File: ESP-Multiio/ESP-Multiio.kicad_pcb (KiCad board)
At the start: 2 copper layers, 75 x 59 mm, 50 parts, among them J1 Conn_01x10, Q1 BC337, SW1 SW_SPDT_MSM, SW2 SW_SPDT_MSM, SW3 SW_SPDT_MSM, SW4 SW_SPDT_MSM, U1 WeMos_D1_mini, U2 MCP23017_SP, U4 TSOP1838

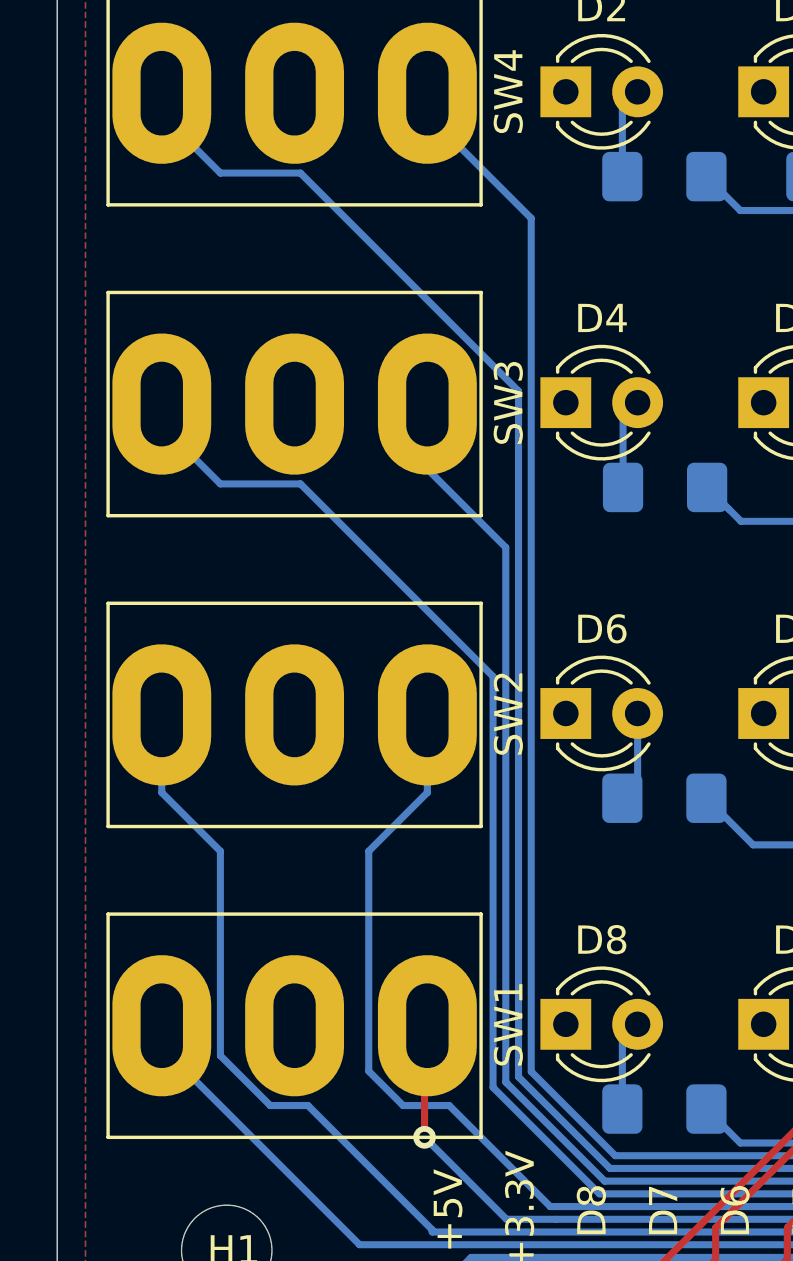
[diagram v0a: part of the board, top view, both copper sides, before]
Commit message: more 3.3V fill
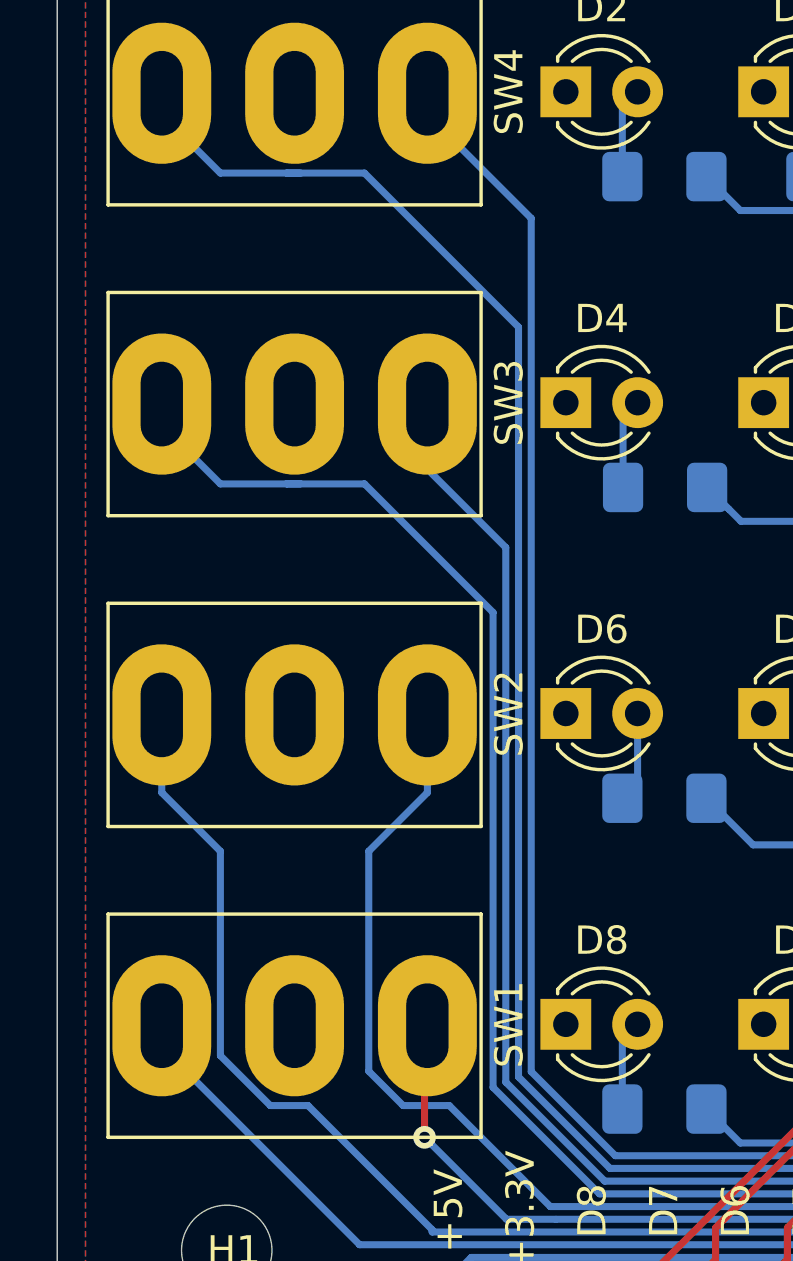
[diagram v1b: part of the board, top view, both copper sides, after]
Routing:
- net /GPB6: track 100.9 -> 102.7 mm
- net /GPB4: track 94.2 -> 96.0 mm
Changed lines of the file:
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@@
     (thickness 1.6)
     (drawings 51)
-    (tracks 363)
+    (tracks 367)
     (zones 0)
     (modules 50)
@@
     (add_net "Net-(Q1-Pad1)")
     (add_net "Net-(Q1-Pad2)")
-    (add_net "Net-(U2-Pad11)")
-    (add_net "Net-(U2-Pad14)")
     (add_net SCL)
     (add_net SDA)
@@
   (segment (start 80.7 51.8) (end 80.7 51.05) (width 0.25) (layer B.Cu) (net 42))
   (segment (start 82.77501 53.87501) (end 80.7 51.8) (width 0.25) (layer B.Cu) (net 42))
-  (segment (start 92.424972 75.234892) (end 92.424972 60.690465) (width 0.25) (layer B.Cu) (net 42))
+  (segment (start 87.87501 53.87501) (end 85.12499 53.87501) (width 0.25) (layer B.Cu) (net 42))
+  (segment (start 92.424972 75.234892) (end 92.424972 58.424972) (width 0.25) (layer B.Cu) (net 42))
+  (segment (start 92.424972 58.424972) (end 87.87501 53.87501) (width 0.25) (layer B.Cu) (net 42))
   (segment (start 96.19013 79.00005) (end 92.424972 75.234892) (width 0.25) (layer B.Cu) (net 42))
-  (segment (start 112.61259 75.80874) (end 109.42128 79.00005) (width 0.25) (layer B.Cu) (net 42))
+  (segment (start 109.42128 79.00005) (end 96.19013 79.00005) (width 0.25) (layer B.Cu) (net 42))
+  (segment (start 112.61259 68.836406) (end 112.61259 75.80874) (width 0.25) (layer B.Cu) (net 42))
+  (segment (start 85.12499 53.87501) (end 82.77501 53.87501) (width 0.25) (layer B.Cu) (net 42))
+  (segment (start 85.609517 53.87501) (end 85.12499 53.87501) (width 0.25) (layer B.Cu) (net 42))
+  (segment (start 118.065994 64.42501) (end 117.023986 64.42501) (width 0.25) (layer B.Cu) (net 42))
   (segment (start 135.84 45.62) (end 135.040001 46.419999) (width 0.25) (layer B.Cu) (net 42))
+  (segment (start 112.61259 75.80874) (end 109.42128 79.00005) (width 0.25) (layer B.Cu) (net 42))
   (segment (start 135.040001 46.419999) (end 135.040001 47.451003) (width 0.25) (layer B.Cu) (net 42))
-  (segment (start 85.609517 53.87501) (end 82.77501 53.87501) (width 0.25) (layer B.Cu) (net 42))
-  (segment (start 135.040001 47.451003) (end 118.065994 64.42501) (width 0.25) (layer B.Cu) (net 42))
   (segment (start 117.023986 64.42501) (end 112.61259 68.836406) (width 0.25) (layer B.Cu) (net 42))
-  (segment (start 92.424972 60.690465) (end 85.609517 53.87501) (width 0.25) (layer B.Cu) (net 42))
-  (segment (start 118.065994 64.42501) (end 117.023986 64.42501) (width 0.25) (layer B.Cu) (net 42))
-  (segment (start 109.42128 79.00005) (end 96.19013 79.00005) (width 0.25) (layer B.Cu) (net 42))
-  (segment (start 112.61259 68.836406) (end 112.61259 75.80874) (width 0.25) (layer B.Cu) (net 42))
+  (segment (start 135.040001 47.451003) (end 118.065994 64.42501) (width 0.25) (layer B.Cu) (net 42))
   (segment (start 92.874981 75.048491) (end 92.874981 56.124981) (width 0.25) (layer B.Cu) (net 43))
   (segment (start 92.874981 56.124981) (end 90 53.25) (width 0.25) (layer B.Cu) (net 43))
@@
   (segment (start 112.16258 66.746416) (end 117.023986 61.88501) (width 0.25) (layer B.Cu) (net 43))
   (segment (start 82.77501 42.87501) (end 80.7 40.8) (width 0.25) (layer B.Cu) (net 44))
-  (segment (start 93.32499 50.590483) (end 85.609517 42.87501) (width 0.25) (layer B.Cu) (net 44))
-  (segment (start 96.56293 78.10003) (end 93.32499 74.86209) (width 0.25) (layer B.Cu) (net 44))
-  (segment (start 93.32499 74.86209) (end 93.32499 50.590483) (width 0.25) (layer B.Cu) (net 44))
+  (segment (start 80.7 40.8) (end 80.7 40.05) (width 0.25) (layer B.Cu) (net 44))
+  (segment (start 87.87501 42.87501) (end 85.12499 42.87501) (width 0.25) (layer B.Cu) (net 44))
+  (segment (start 93.32499 74.86209) (end 93.32499 48.32499) (width 0.25) (layer B.Cu) (net 44))
   (segment (start 109.04848 78.10003) (end 96.56293 78.10003) (width 0.25) (layer B.Cu) (net 44))
+  (segment (start 111.71257 64.656426) (end 111.71257 75.43594) (width 0.25) (layer B.Cu) (net 44))
+  (segment (start 117.023986 59.34501) (end 111.71257 64.656426) (width 0.25) (layer B.Cu) (net 44))
+  (segment (start 85.12499 42.87501) (end 82.77501 42.87501) (width 0.25) (layer B.Cu) (net 44))
+  (segment (start 118.065994 59.34501) (end 117.023986 59.34501) (width 0.25) (layer B.Cu) (net 44))
+  (segment (start 96.56293 78.10003) (end 93.32499 74.86209) (width 0.25) (layer B.Cu) (net 44))
+  (segment (start 129.960001 46.419999) (end 129.960001 47.451003) (width 0.25) (layer B.Cu) (net 44))
+  (segment (start 85.609517 42.87501) (end 85.12499 42.87501) (width 0.25) (layer B.Cu) (net 44))
   (segment (start 111.71257 75.43594) (end 109.04848 78.10003) (width 0.25) (layer B.Cu) (net 44))
   (segment (start 130.76 45.62) (end 129.960001 46.419999) (width 0.25) (layer B.Cu) (net 44))
+  (segment (start 93.32499 48.32499) (end 87.87501 42.87501) (width 0.25) (layer B.Cu) (net 44))
   (segment (start 129.960001 47.451003) (end 118.065994 59.34501) (width 0.25) (layer B.Cu) (net 44))
-  (segment (start 80.7 40.8) (end 80.7 40.05) (width 0.25) (layer B.Cu) (net 44))
-  (segment (start 129.960001 46.419999) (end 129.960001 47.451003) (width 0.25) (layer B.Cu) (net 44))
-  (segment (start 111.71257 64.656426) (end 111.71257 75.43594) (width 0.25) (layer B.Cu) (net 44))
-  (segment (start 85.609517 42.87501) (end 82.77501 42.87501) (width 0.25) (layer B.Cu) (net 44))
-  (segment (start 118.065994 59.34501) (end 117.023986 59.34501) (width 0.25) (layer B.Cu) (net 44))
-  (segment (start 117.023986 59.34501) (end 111.71257 64.656426) (width 0.25) (layer B.Cu) (net 44))
   (segment (start 90.1 40.8) (end 90.1 40.05) (width 0.25) (layer B.Cu) (net 45))
   (segment (start 93.774999 44.474999) (end 90.1 40.8) (width 0.25) (layer B.Cu) (net 45))
